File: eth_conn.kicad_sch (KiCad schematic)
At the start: 25 parts, among them J1 RJ45

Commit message: did 3v3 reg
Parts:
- C36, C37: footprint (none) -> Capacitor_SMD:C_0402_1005Metric
- R29, R30, R31, R32, R33, R34: footprint (none) -> Resistor_SMD:R_0402_1005Metric
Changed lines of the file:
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@@
 			)
 		)
-		(property "Footprint" ""
+		(property "Footprint" "Resistor_SMD:R_0402_1005Metric"
 			(at 203.962 158.75 90)
 			(effects
@@
 			)
 		)
-		(property "Footprint" ""
+		(property "Footprint" "Capacitor_SMD:C_0402_1005Metric"
 			(at 169.8752 160.02 0)
 			(effects
@@
 			)
 		)
-		(property "Footprint" ""
+		(property "Footprint" "Resistor_SMD:R_0402_1005Metric"
 			(at 279.4 140.208 90)
 			(effects
@@
 			)
 		)
-		(property "Footprint" ""
+		(property "Footprint" "Resistor_SMD:R_0402_1005Metric"
 			(at 279.4 144.272 90)
 			(effects
@@
 			)
 		)
-		(property "Footprint" ""
+		(property "Footprint" "Capacitor_SMD:C_0402_1005Metric"
 			(at 155.9052 160.02 0)
 			(effects
@@
 			)
 		)
-		(property "Footprint" ""
+		(property "Footprint" "Resistor_SMD:R_0402_1005Metric"
 			(at 276.352 158.75 90)
 			(effects
@@
 			)
 		)
-		(property "Footprint" ""
+		(property "Footprint" "Resistor_SMD:R_0402_1005Metric"
 			(at 214.122 158.75 90)
 			(effects
@@
 			)
 		)
-		(property "Footprint" ""
+		(property "Footprint" "Resistor_SMD:R_0402_1005Metric"
 			(at 267.462 158.75 90)
 			(effects

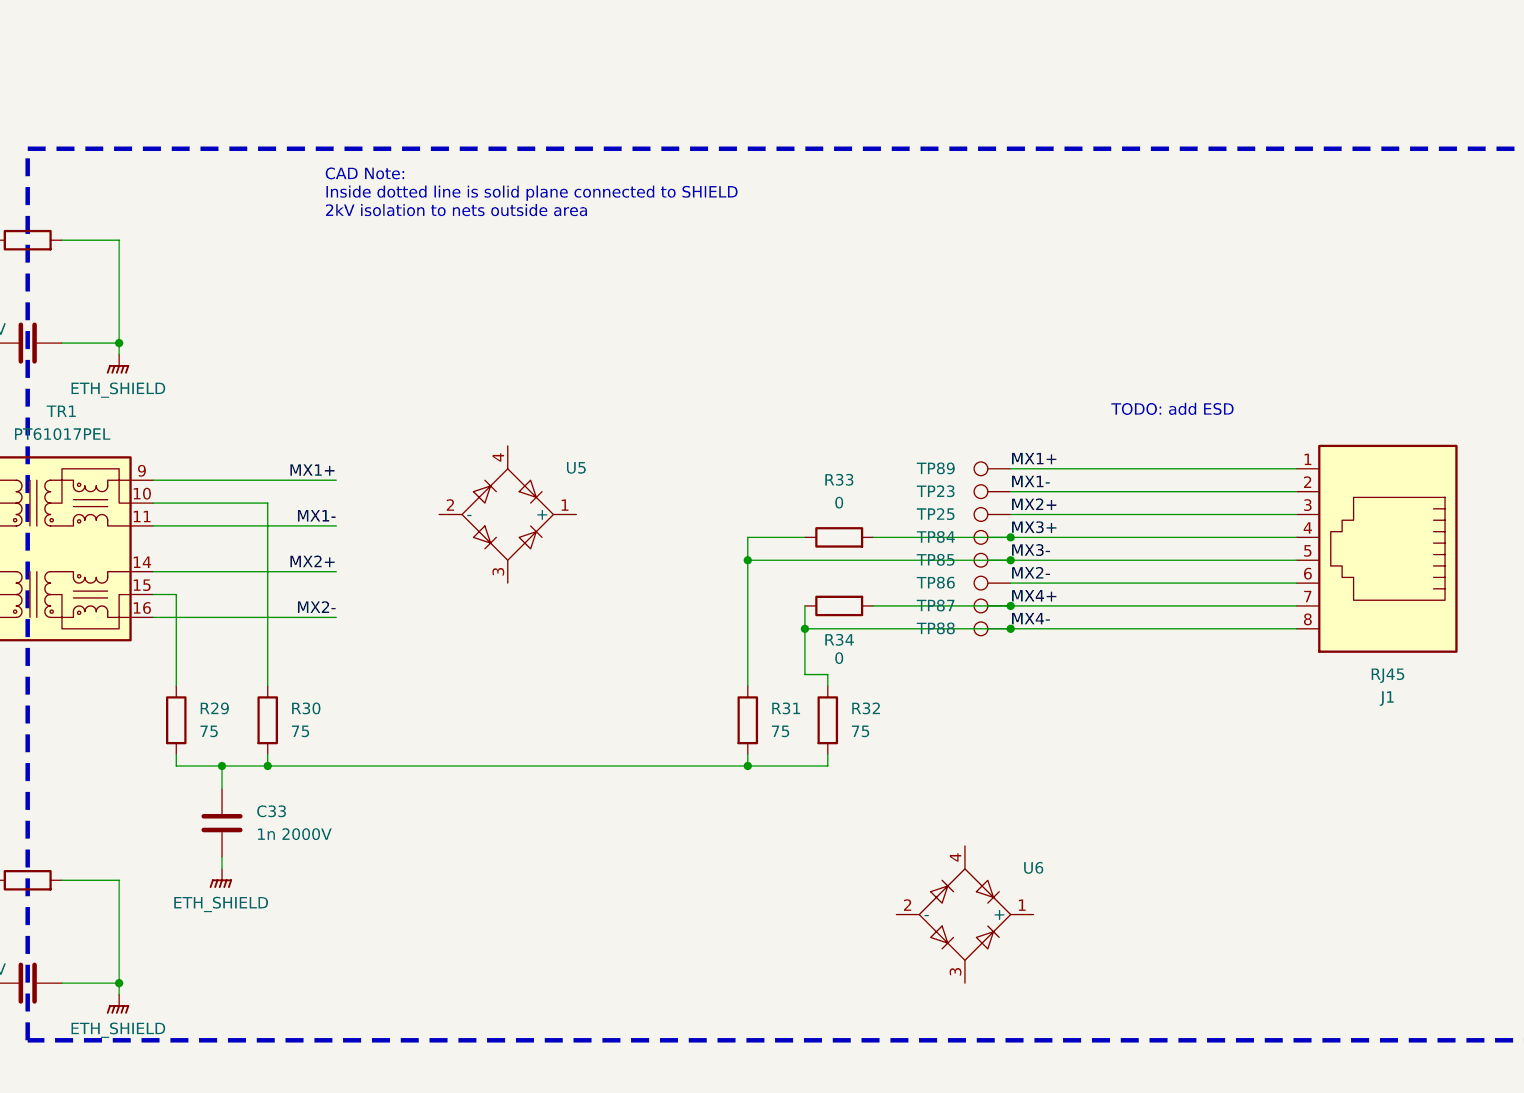
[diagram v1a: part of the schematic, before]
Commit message: stuff
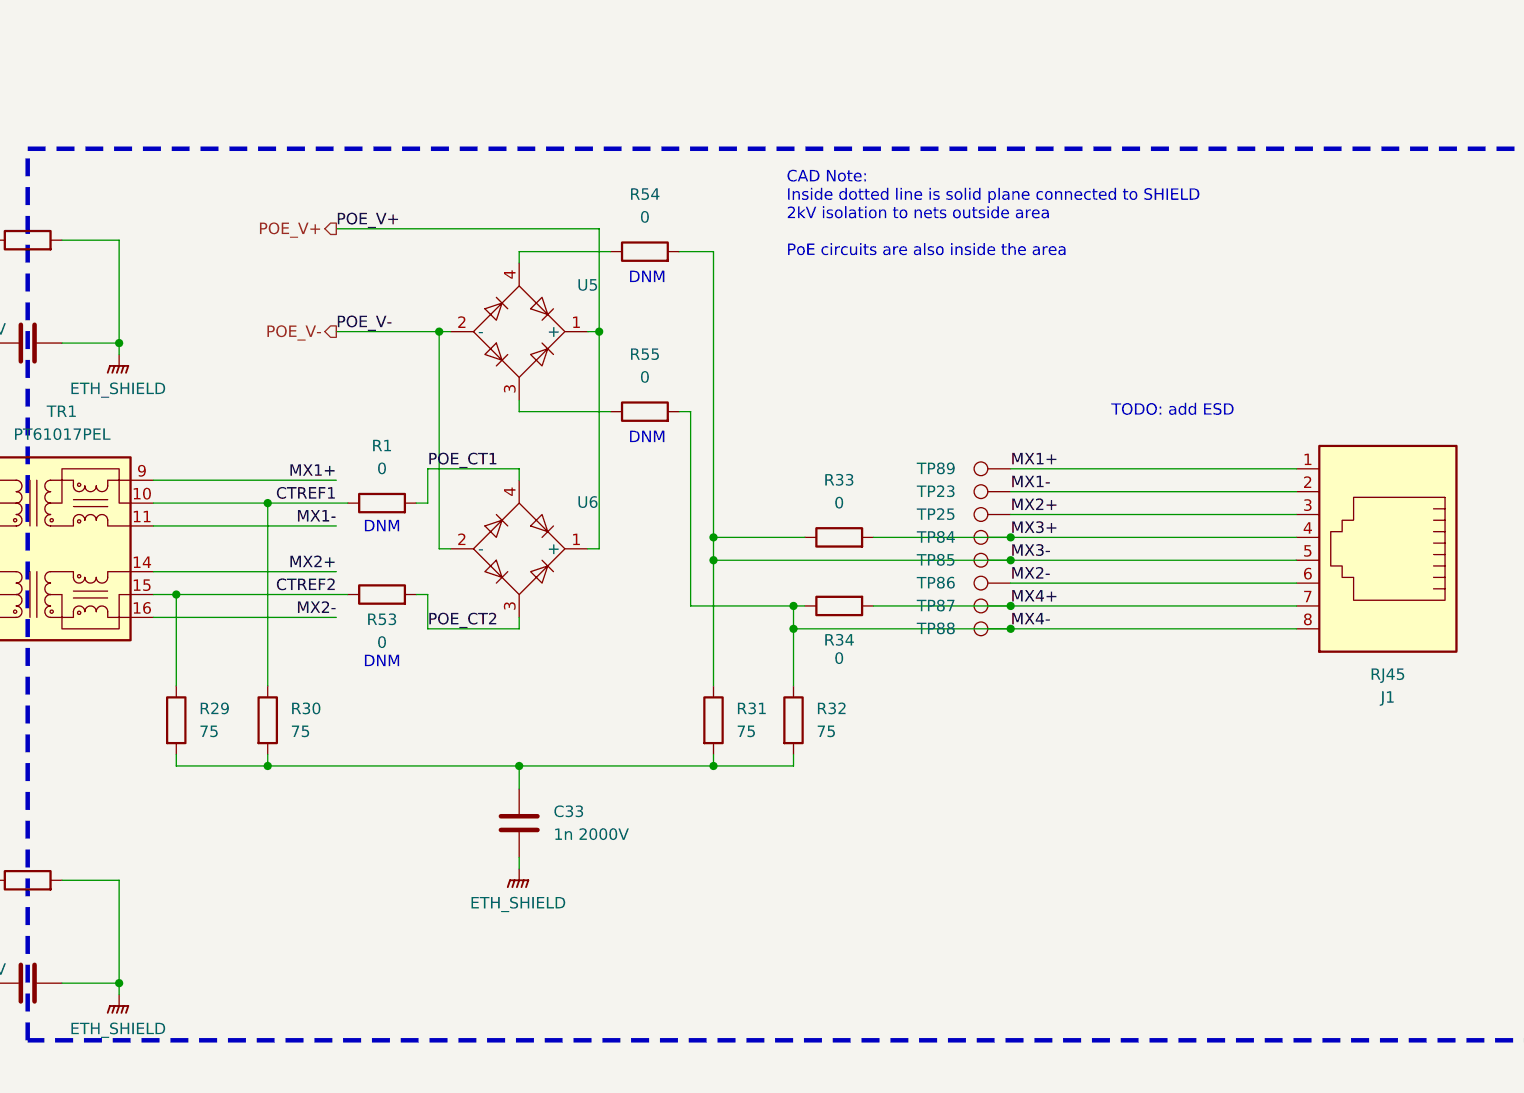
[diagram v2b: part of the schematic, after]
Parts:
- added R1, R53, R54, R55: 0, Resistor_SMD:R_0402_1005Metric, symbol Device:R
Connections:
- net MX3-: now also R54.2
- net MX4-: now also R55.2
- net CTREF2: now reaches R29.1, TR1.15 (C_TX)
- net CTREF2: now also R53.1
- net POE_V+: now reaches U6.1 (+)
- net POE_V+: now also U5.1 (+)
- net POE_V-: now reaches U6.2 (-)
- net POE_V-: now also U5.2 (-)
- net POE_CT2: now reaches U6.3
- net POE_CT2: now also R53.2
- net POE_CT1: now reaches U6.4
- net POE_CT1: now also R1.2
- net at U5.3: now also R55.1
- net at U5.4: now also R54.1
- net CTREF1: now reaches R30.1, TR1.10 (C_RX)
- net CTREF1: now also R1.1
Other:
- note added: "CAD Note: Inside dotted line is solid plane connected to SHIELD 2kV isolation to nets outside area PoE circuits are also inside the area"
- note added: "DNM"
- note removed: "CAD Note: Inside dotted line is solid plane connected to SHIELD 2kV isolation to nets outside area"
- moved on the sheet: C33, R31, R32, U5, U6
